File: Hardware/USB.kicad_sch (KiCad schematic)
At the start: 7 parts, among them J3 USB_C_Receptacle_USB2.0_14P, U3 USBLC6-2SC6, U4 AP2112K-3.3

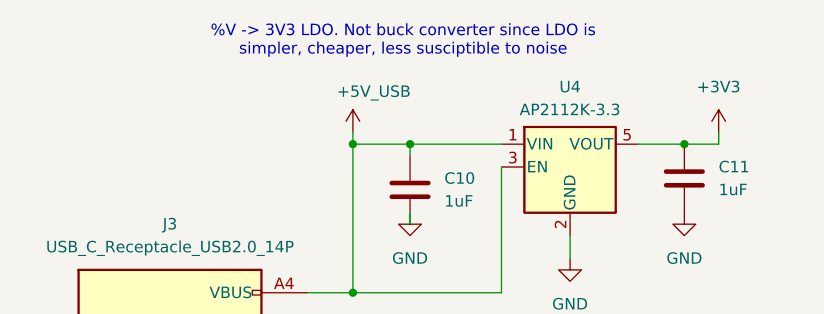
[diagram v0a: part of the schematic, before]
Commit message: Updated: ERC fixes
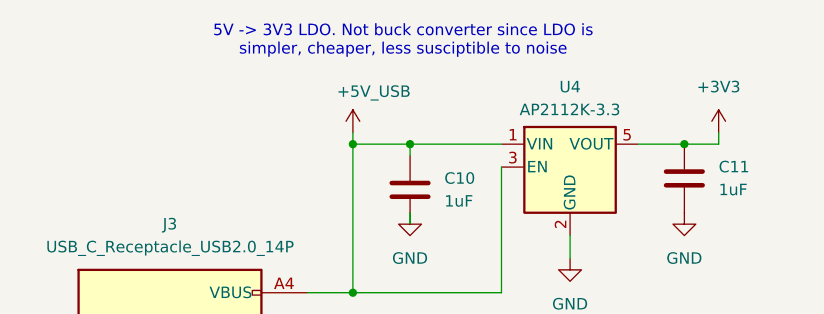
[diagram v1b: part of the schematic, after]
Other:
- note added: "5V -> 3V3 LDO. Not buck converter since LDO is simpler, cheaper, less susciptible to noise"
- note removed: "%V -> 3V3 LDO. Not buck converter since LDO is simpler, cheaper, less susciptible to noise"
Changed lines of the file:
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@@
 	(generator_version "9.0")
 	(paper "A4")
-	(text "%V -> 3V3 LDO. Not buck converter since LDO is \nsimpler, cheaper, less susciptible to noise\n"
+	(text "5V -> 3V3 LDO. Not buck converter since LDO is \nsimpler, cheaper, less susciptible to noise\n"
 		(exclude_from_sim no)
 		(at 105.918 49.53 0)
